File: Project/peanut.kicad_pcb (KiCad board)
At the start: 2 copper layers, 227.9 x 65.3 mm, 70 parts, among them J1 USB_C_Receptacle_USB2.0, SW1 RotaryEncoder_Switch, SW2 SKQGABE010, U1 STM32F072C8Tx, U2 AP2112K-3.3, U3 PRTR5V0U2X

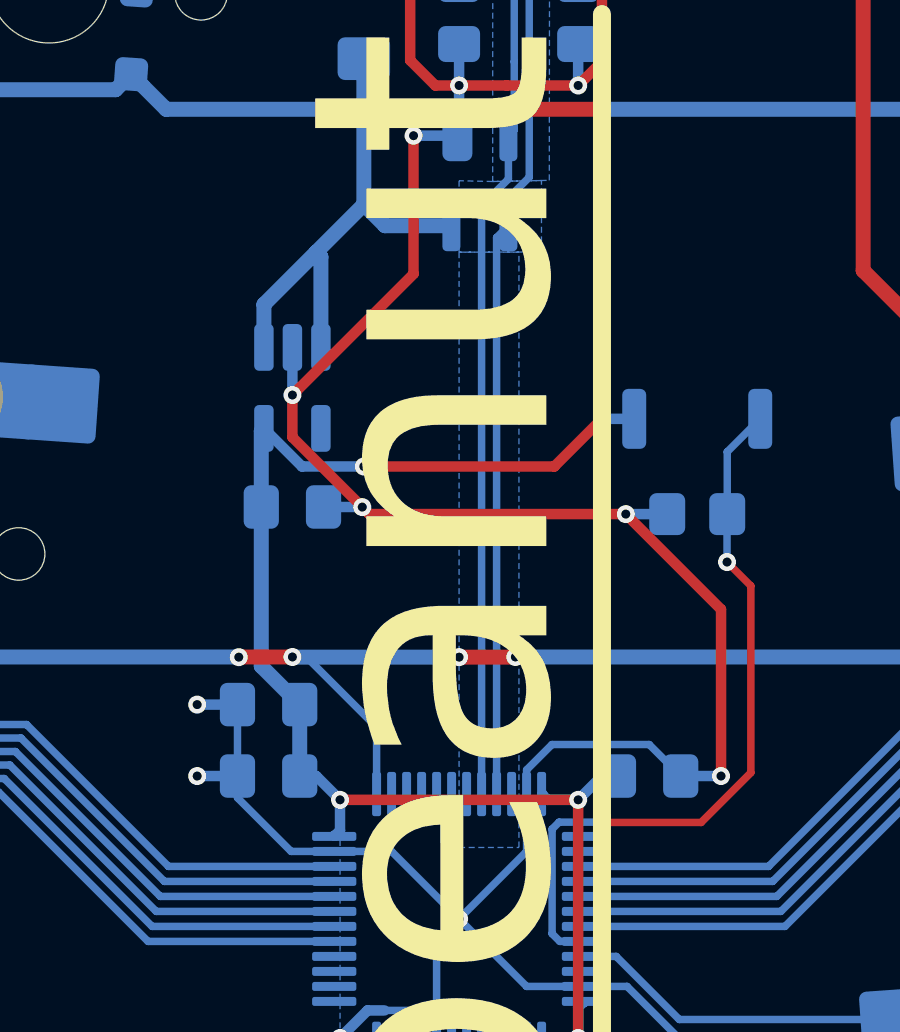
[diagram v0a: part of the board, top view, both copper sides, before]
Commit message: update
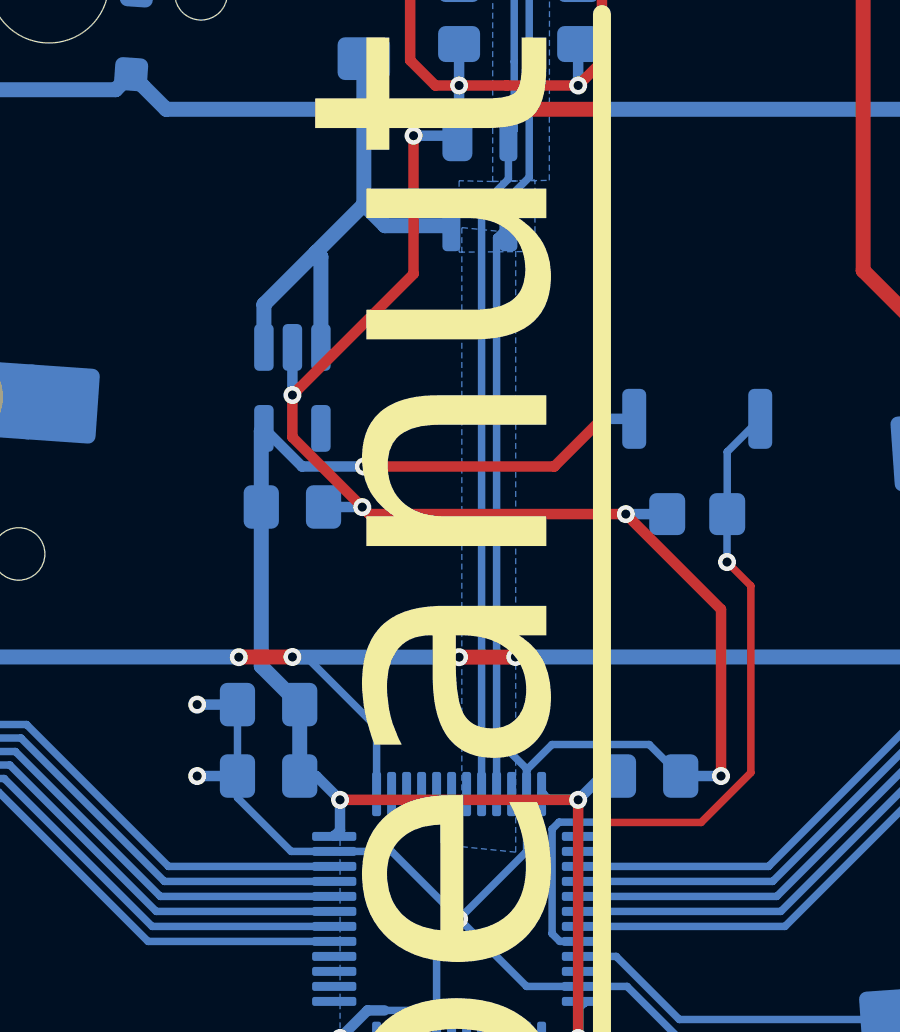
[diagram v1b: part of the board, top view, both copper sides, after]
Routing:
- net GND: track 164.8 -> 166.8 mm
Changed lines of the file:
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@@
 				(xy -11.579411 10.494097) (xy -10.04379 10.54183) (xy -9.995573 11.911438) (xy -9.947356 13.281046)
 				(xy -11.426466 13.281046) (xy -12.905576 13.281046) (xy -13.008477 12.658497) (xy -13.073657 12.088282)
-				(xy -13.110378 11.427351) (xy -13.113205 11.241156) (xy -13.115032 10.446364)
+				(xy -13.110377 11.427351) (xy -13.113205 11.241156) (xy -13.115032 10.446364)
 			)
 			(stroke
@@
 				(xy -24.406226 16.022585) (xy -24.482659 15.024183) (xy -24.587993 13.646557) (xy -24.689776 12.338358)
 				(xy -24.784279 11.145763) (xy -24.867779 10.114952) (xy -24.936551 9.292098) (xy -24.986869 8.72338)
-				(xy -25.008329 8.508169) (xy -25.10623 7.636601) (xy -21.766842 7.636598) (xy -18.427451 7.636601)
+				(xy -25.008329 8.508169) (xy -25.10623 7.636601) (xy -21.766842 7.636597) (xy -18.427451 7.636601)
 				(xy -18.427451 8.63268) (xy -18.42745 9.628758) (xy -20.747483 9.628757) (xy -23.067515 9.628758)
-				(xy -22.993212 10.085294) (xy -22.96006 10.370984) (xy -22.905349 10.937963) (xy -22.833468 11.736512)
+				(xy -22.993212 10.085294) (xy -22.96006 10.370984) (xy -22.905349 10.937963) (xy -22.833469 11.736512)
 				(xy -22.748797 12.716909) (xy -22.655735 13.829433) (xy -22.571994 14.85817) (xy -22.476083 16.028102)
 				(xy -22.385149 17.093548) (xy -22.303431 18.00829) (xy -22.235159 18.72611) (xy -22.184568 19.200795)
@@
 				(xy -20.253169 -3.287291) (xy -20.214704 -4.210653) (xy -20.16635 -5.378311) (xy -20.109307 -6.761115)
 				(xy -20.044774 -8.329912) (xy -19.973955 -10.055551) (xy -19.89805 -11.908882) (xy -19.818259 -13.86075)
-				(xy -19.747491 -15.594977) (xy -19.66629 -17.574174) (xy -19.588214 -19.454383) (xy -19.514387 -21.209627)
+				(xy -19.747492 -15.594977) (xy -19.666289 -17.574174) (xy -19.588214 -19.454383) (xy -19.514387 -21.209627)
 				(xy -19.445945 -22.813917) (xy -19.384032 -24.241272) (xy -19.329782 -25.465708) (xy -19.284333 -26.46124)
 				(xy -19.248826 -27.201884) (xy -19.224395 -27.661658) (xy -19.212429 -27.814672) (xy -19.044283 -27.824794)
@@
 				(xy -24.867779 10.114952) (xy -24.936551 9.292098) (xy -24.986869 8.72338) (xy -25.008329 8.50817)
 				(xy -25.10623 7.636601) (xy -21.766841 7.6366) (xy -18.427451 7.636601) (xy -18.427451 8.63268)
-				(xy -18.427451 9.628758) (xy -20.747483 9.628757) (xy -23.067512 9.628758) (xy -22.993212 10.085294)
+				(xy -18.427451 9.628758) (xy -20.747483 9.628757) (xy -23.067511 9.628758) (xy -22.993212 10.085294)
 				(xy -22.96006 10.370984) (xy -22.905349 10.937963) (xy -22.833466 11.736511) (xy -22.748798 12.716909)
-				(xy -22.655735 13.829433) (xy -22.571994 14.85817) (xy -22.476086 16.028102) (xy -22.38515 17.093548)
+				(xy -22.655735 13.829433) (xy -22.571994 14.85817) (xy -22.476087 16.028102) (xy -22.38515 17.093548)
 				(xy -22.303431 18.00829) (xy -22.235159 18.726111) (xy -22.184567 19.200795) (xy -22.157619 19.382026)
 				(xy -22.086811 19.41267) (xy -21.885926 19.440346) (xy -21.540894 19.465183) (xy -21.037644 19.487313)
@@
 				(xy -4.397536 -28.286389) (xy -3.003109 -28.31557) (xy -1.715571 -28.333875) (xy -0.482445 -28.341305)
 				(xy 0.748747 -28.337861) (xy 2.030481 -28.323545) (xy 3.415236 -28.298358) (xy 4.955487 -28.262302)
-				(xy 6.703713 -28.215378) (xy 8.712389 -28.157587) (xy 9.510595 -28.134086) (xy 11.285613 -28.080495)
+				(xy 6.703713 -28.215378) (xy 8.712389 -28.157587) (xy 9.510595 -28.134086) (xy 11.285614 -28.080495)
 				(xy 12.960314 -28.027701) (xy 14.505523 -27.976775) (xy 15.892046 -27.928783) (xy 17.090695 -27.884797)
 				(xy 18.072281 -27.845883) (xy 18.807614 -27.813112) (xy 19.267507 -27.787551) (xy 19.422493 -27.771132)
@@
 		(fp_arc
 			(start -4.864823 3.20022)
-			(mid -4.718372 2.846671)
+			(mid -4.718373 2.846672)
 			(end -4.364825 2.700219)
 			(stroke
@@
 		(fp_arc
 			(start -4.864823 3.20022)
-			(mid -4.718372 2.846671)
+			(mid -4.718373 2.846672)
 			(end -4.364825 2.700219)
 			(stroke
@@
 		(fp_arc
 			(start -4.864823 3.20022)
-			(mid -4.718372 2.846671)
+			(mid -4.718373 2.846672)
 			(end -4.364825 2.700219)
 			(stroke
@@
 		(fp_arc
 			(start -4.864823 3.20022)
-			(mid -4.718372 2.846671)
+			(mid -4.718373 2.846672)
 			(end -4.364825 2.700219)
 			(stroke
@@
 		(fp_arc
 			(start -4.864823 3.20022)
-			(mid -4.718372 2.846671)
+			(mid -4.718373 2.846672)
 			(end -4.364825 2.700219)
 			(stroke
@@
 		(fp_arc
 			(start -4.864823 3.20022)
-			(mid -4.718372 2.846671)
+			(mid -4.718373 2.846672)
 			(end -4.364825 2.700219)
 			(stroke
@@
 		(fp_arc
 			(start -4.864823 3.20022)
-			(mid -4.718372 2.846671)
+			(mid -4.718373 2.846672)
 			(end -4.364825 2.700219)
 			(stroke
@@
 		(fp_arc
 			(start -4.864823 3.20022)
-			(mid -4.718372 2.846671)
+			(mid -4.718373 2.846672)
 			(end -4.364825 2.700219)
 			(stroke
@@
 		(fp_arc
 			(start -4.864823 3.20022)
-			(mid -4.718372 2.846671)
+			(mid -4.718373 2.846672)
 			(end -4.364825 2.700219)
 			(stroke
@@
 		(fp_arc
 			(start -4.864823 3.20022)
-			(mid -4.718372 2.846671)
+			(mid -4.718373 2.846672)
 			(end -4.364825 2.700219)
 			(stroke
@@
 		(fp_arc
 			(start -4.864823 3.20022)
-			(mid -4.718372 2.846671)
+			(mid -4.718373 2.846672)
 			(end -4.364825 2.700219)
 			(stroke
@@
 		(fp_arc
 			(start -4.864823 3.20022)
-			(mid -4.718372 2.846671)
+			(mid -4.718373 2.846672)
 			(end -4.364825 2.700219)
 			(stroke
@@
 	)
 	(segment
+		(start 150.760469 71.203708)
+		(end 150.994261 71.4375)
+		(width 0.25)
+		(layer "B.Cu")
+		(net 44)
+	)
+	(segment
 		(start 148.43125 91.025)
 		(end 147.93125 91.025)
@@
 	)
 	(segment
+		(start 156.2375 80.76875)
+		(end 156.2375 79.925)
+		(width 0.25)
+		(layer "B.Cu")
+		(net 44)
+	)
+	(segment
 		(start 152.17 50.0825)
 		(end 151.255 49.1675)
@@
 	)
 	(segment
+		(start 156.2375 79.925)
+		(end 155.6875 79.375)
+		(width 0.25)
+		(layer "B.Cu")
+		(net 44)
+	)
+	(segment
 		(start 146.6 80.16875)
 		(end 145.25625 80.16875)
@@
 			(thermal_gap 0.5)
 			(thermal_bridge_width 0.5)
+			(island_removal_mode 1)
+			(island_area_min 10)
 		)
 		(polygon
 			(pts
-				(xy 153.9875 62.70625) (xy 153.9875 82.55) (xy 155.982853 82.55) (xy 155.982853 62.70625)
+				(xy 154.078616 61.88673) (xy 154.078616 82.52423) (xy 155.87491 82.706464) (xy 155.87491 62.068964)
 			)
 		)
@@
 		(polygon
 			(pts
-				(xy 155.106665 60.351033) (xy 153.9875 60.325) (xy 153.9875 62.70625) (xy 156.733215 62.699873)
-				(xy 156.733215 60.318623)
+				(xy 155.106665 60.351033) (xy 153.9875 60.325) (xy 153.9875 62.70625) (xy 156.516272 62.68199) (xy 156.516272 60.30074)
 			)
 		)

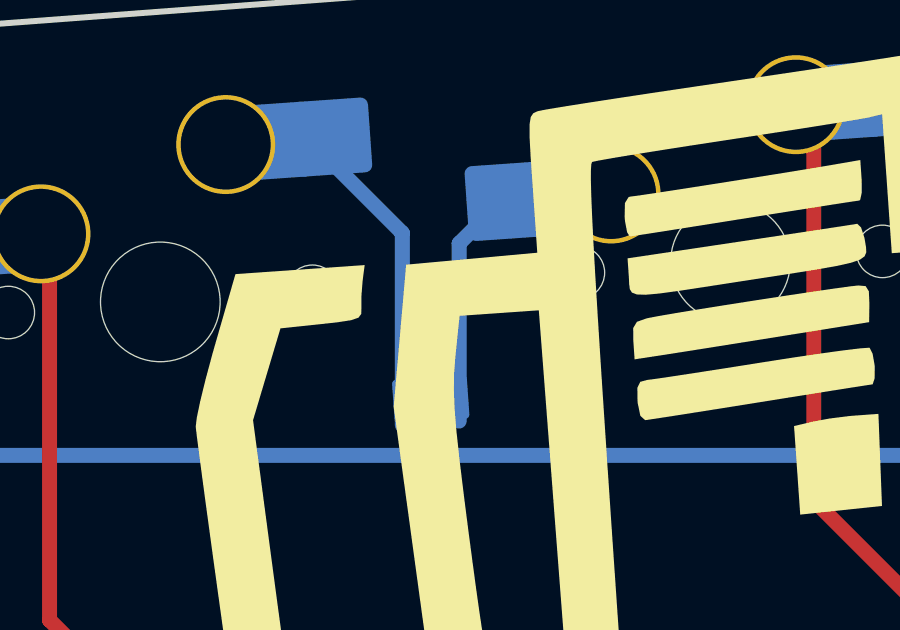
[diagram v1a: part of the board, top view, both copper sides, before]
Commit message: firmware
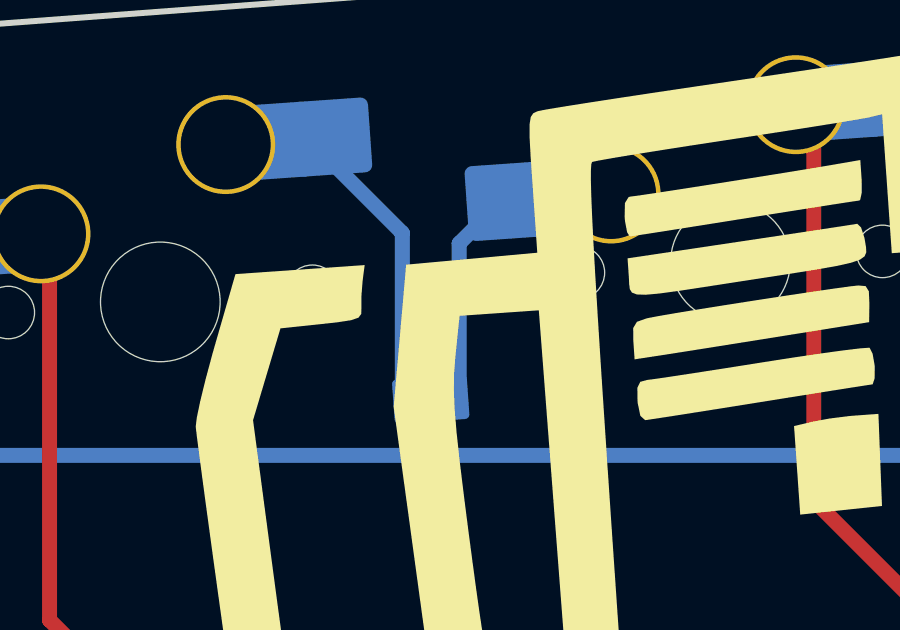
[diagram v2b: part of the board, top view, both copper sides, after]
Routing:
- net Net-(D9-A2): track 11.0 -> 10.2 mm
- net Net-(D9-A1): track 14.1 -> 13.3 mm
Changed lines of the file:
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@@
 				(xy -25.008329 8.508169) (xy -25.10623 7.636601) (xy -21.766842 7.636597) (xy -18.427451 7.636601)
 				(xy -18.427451 8.63268) (xy -18.42745 9.628758) (xy -20.747483 9.628757) (xy -23.067515 9.628758)
-				(xy -22.993212 10.085294) (xy -22.96006 10.370984) (xy -22.905349 10.937963) (xy -22.833469 11.736512)
+				(xy -22.993212 10.085294) (xy -22.96006 10.370984) (xy -22.905349 10.937963) (xy -22.83347 11.736512)
 				(xy -22.748797 12.716909) (xy -22.655735 13.829433) (xy -22.571994 14.85817) (xy -22.476083 16.028102)
 				(xy -22.385149 17.093548) (xy -22.303431 18.00829) (xy -22.235159 18.72611) (xy -22.184568 19.200795)
@@
 				(xy -24.867779 10.114952) (xy -24.936551 9.292098) (xy -24.986869 8.72338) (xy -25.008329 8.50817)
 				(xy -25.10623 7.636601) (xy -21.766841 7.6366) (xy -18.427451 7.636601) (xy -18.427451 8.63268)
-				(xy -18.427451 9.628758) (xy -20.747483 9.628757) (xy -23.067511 9.628758) (xy -22.993212 10.085294)
+				(xy -18.427451 9.628758) (xy -20.747483 9.628757) (xy -23.06751 9.628758) (xy -22.993212 10.085294)
 				(xy -22.96006 10.370984) (xy -22.905349 10.937963) (xy -22.833466 11.736511) (xy -22.748798 12.716909)
 				(xy -22.655735 13.829433) (xy -22.571994 14.85817) (xy -22.476087 16.028102) (xy -22.38515 17.093548)
@@
 	)
 	(segment
-		(start 195.139494 46.501464)
-		(end 195.387129 46.253829)
+		(start 198.218167 49.084867)
+		(end 198.218167 54.693552)
 		(width 0.5)
 		(layer "B.Cu")
@@
 	)
 	(segment
-		(start 198.218167 55.487302)
-		(end 198.218167 49.084867)
+		(start 195.139494 46.501464)
+		(end 195.387129 46.253829)
 		(width 0.5)
 		(layer "B.Cu")
@@
 	)
 	(segment
-		(start 200.113539 55.354765)
-		(end 200.113539 49.434137)
+		(start 200.113539 49.434137)
+		(end 200.113539 54.561015)
 		(width 0.5)
 		(layer "B.Cu")
@@
 	(segment
 		(start 201.398306 48.14937)
-		(end 201.15067 48.397006)
-		(width 0.5)
-		(layer "B.Cu")
-		(net 17)
-	)
-	(segment
-		(start 200.113539 49.434137)
-		(end 201.15067 48.397006)
+		(end 200.113539 49.434137)
 		(width 0.5)
 		(layer "B.Cu")
